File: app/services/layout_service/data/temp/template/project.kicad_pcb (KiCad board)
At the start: 2 copper layers, 58 parts, among them J1 CUI_PJ-044A, J2 61300611121, J3 61300311121, M1 MIC_ICS-40720, Q1 SOT-23_DIO, Q2 SOT-323_DIO, U1 SOT25_DIO, U2 SOT-23_MC_MCH, U3 LQFP64-10x10mm, U4 MR25H40CDC_EVS, U5 8L_USON_2X3_ISI, U6 1351-01_NXP, U7 MC3635_MEM, U8 BMX160_BOS, X1 XTAL_NX5032GA-16.000M-STD-CSU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

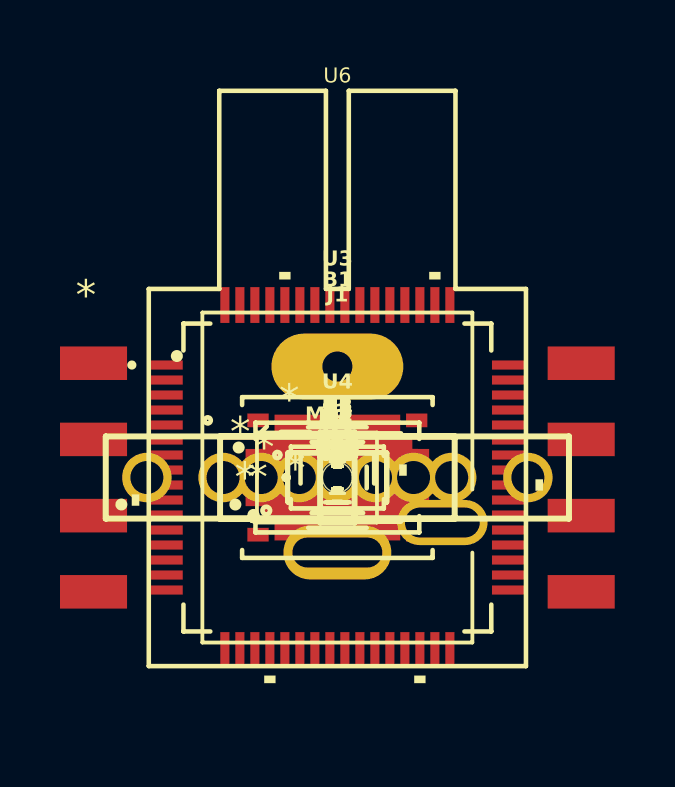
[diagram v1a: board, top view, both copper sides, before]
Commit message: 流程适配完成-v1.0
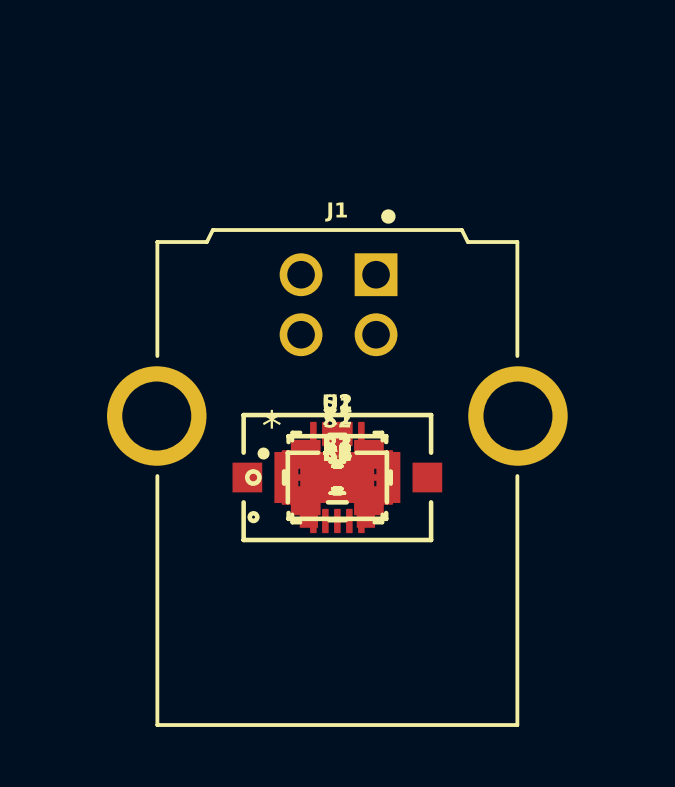
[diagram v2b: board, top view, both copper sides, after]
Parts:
- removed B1: Battery_CR1225, Battery_CR1225
- removed C10, C11, C12, C13, C14, C15, C9: CAPC1005X55N, 0402C
- removed C16, C17: YAG_CC0603_YAG, YAG_CC0603_YAG
- removed C18: CAP_CL10A105KB8NNN_SAM, CAP_CL10A105KB8NNN_SAM
- removed C19: 0402_AVX, 0402_AVX
- removed C20, C22: CAP_0402_SAM, CAP_0402_SAM
- removed C21, C24, C25, C26: C_0603_1608Metric, C_0603_1608Metric
- removed C23: C_0402_1005Metric, C_0402_1005Metric
- removed D1: SOD-123_ONS, SOD-123_ONS
- removed D2: SDO_CFP5_SOD128_NEX, SDO_CFP5_SOD128_NEX
- removed I1: SOT95P285X113-3N, SOT95P285X113-3N
- removed J2: 61300611121, 61300611121
- removed J3: 61300311121, 61300311121
- removed M1: MIC_ICS-40720, MIC_ICS-40720
- removed Q1: SOT-23_DIO, SOT-23_DIO
- removed Q2: SOT-323_DIO, SOT-323_DIO
- removed R10, R11, R12, R9: RES_ERJ-2GEJ103X, 0402R
- removed R8: R_0402_1005Metric, R_0402_1005Metric
- removed U3: LQFP64-10x10mm, STM32F103RET6
- removed U4: MR25H40CDC_EVS, MR25H40CDC_EVS
- removed U5: 8L_USON_2X3_ISI, 8L_USON_2X3_ISI
- removed U6: 1351-01_NXP, 1351-01_NXP
- removed U7: MC3635_MEM, MC3635_MEM
- removed U8: BMX160_BOS, BMX160_BOS
- added L1: LED_LTST-C191KRKT_LTO, LED_LTST-C191KRKT_LTO, F.Cu at (0.00, 0.00)
- added S2: B3U-1000P, B3U-1000P, F.Cu at (0.00, 0.00)
- C5: value SOT23-3_LTF -> C_0402_1005Metric; footprint SOT23-3_LTF -> C_0402_1005Metric
- C6, C7, C8: value CAPC1005X55N -> C_0402_1005Metric; footprint 0402C -> C_0402_1005Metric
- J1: value CUI_PJ-044A -> ASSMANN_AU-Y1007; footprint CUI_PJ-044A -> ASSMANN_AU-Y1007
- R1: value R_0402_1005Metric -> R_0603_1608Metric; footprint R_0402_1005Metric -> R_0603_1608Metric
- R2: value R_0402_1005Metric -> RC0402N_PAN; footprint R_0402_1005Metric -> RC0402N_PAN
- S1: value SW_KMR221GLFS -> SW_25816_WRE; footprint KMR221GLFS -> SW_25816_WRE
- U1: value SOT25_DIO -> SOT-23_MC_MCH; footprint SOT25_DIO -> SOT-23_MC_MCH
- U2: value SOT-23_MC_MCH -> QFN40P300X300X90-21N; footprint SOT-23_MC_MCH -> QFN40P300X300X90-21N
- X1: value XTAL_NX5032GA-16.000M-STD-CSU-2_NDK -> CRYSTAL_ABM8G_ABR; footprint NX5032GA_16_000M_STD_CSU_2 -> ABM8G_12_000MHZ_B4Y_T
